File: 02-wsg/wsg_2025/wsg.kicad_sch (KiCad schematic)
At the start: 4 parts, among them J1 Conn_02x04_Counter_Clockwise, P1 USB_C_Plug_USB2.0, U5 ESP32-C6

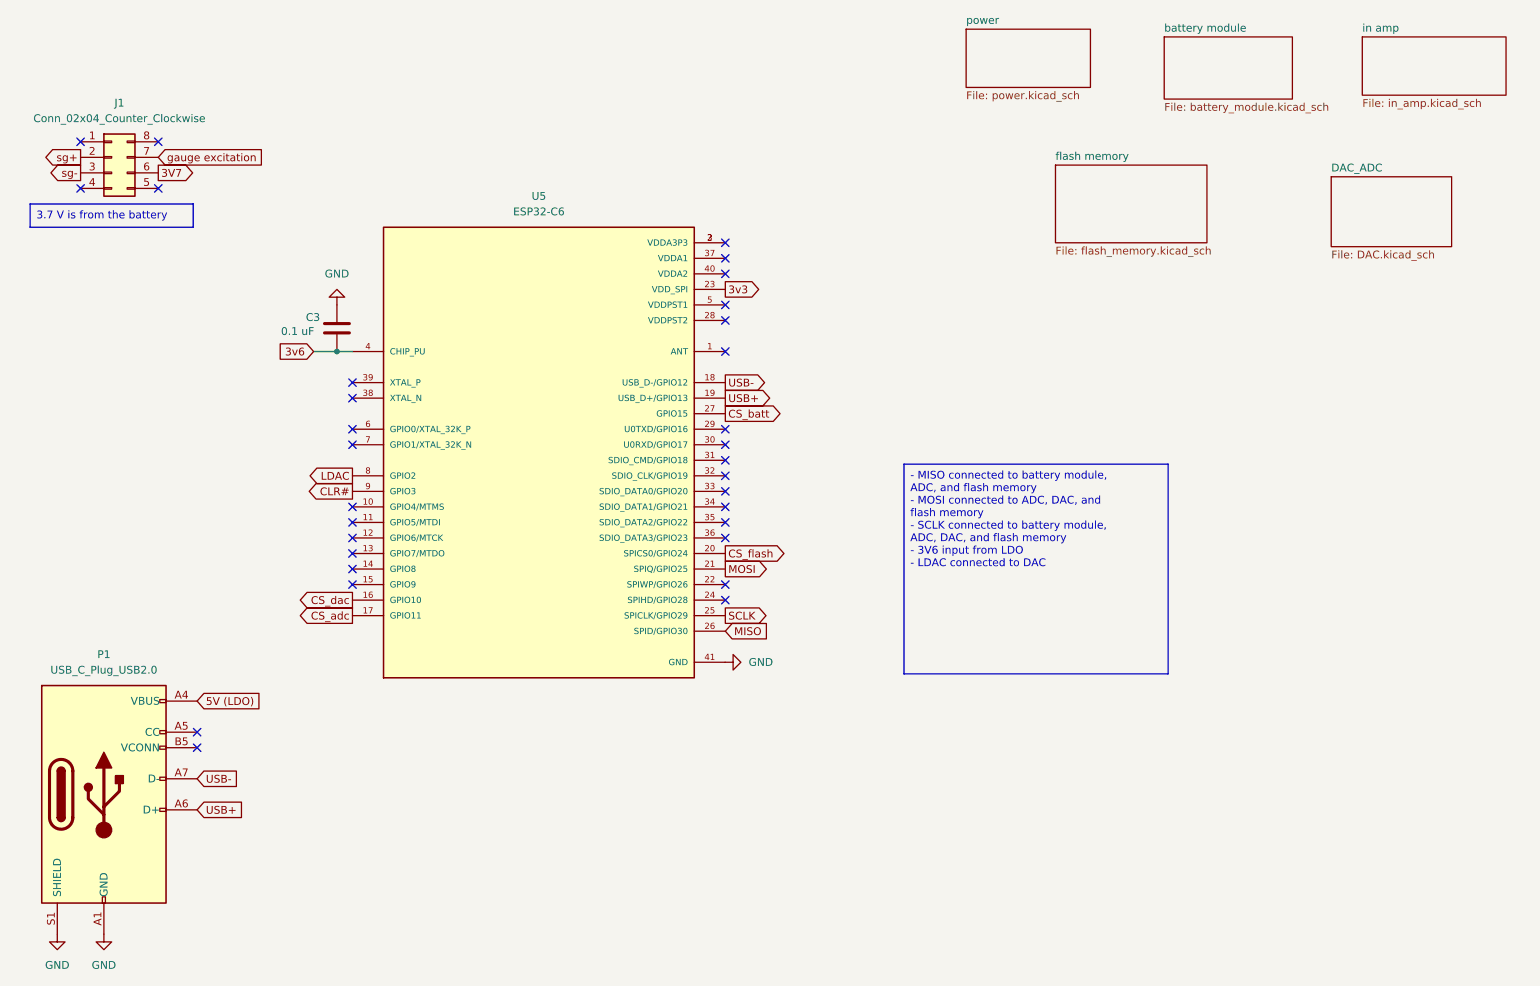
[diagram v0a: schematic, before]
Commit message: new wsg schem - not complete
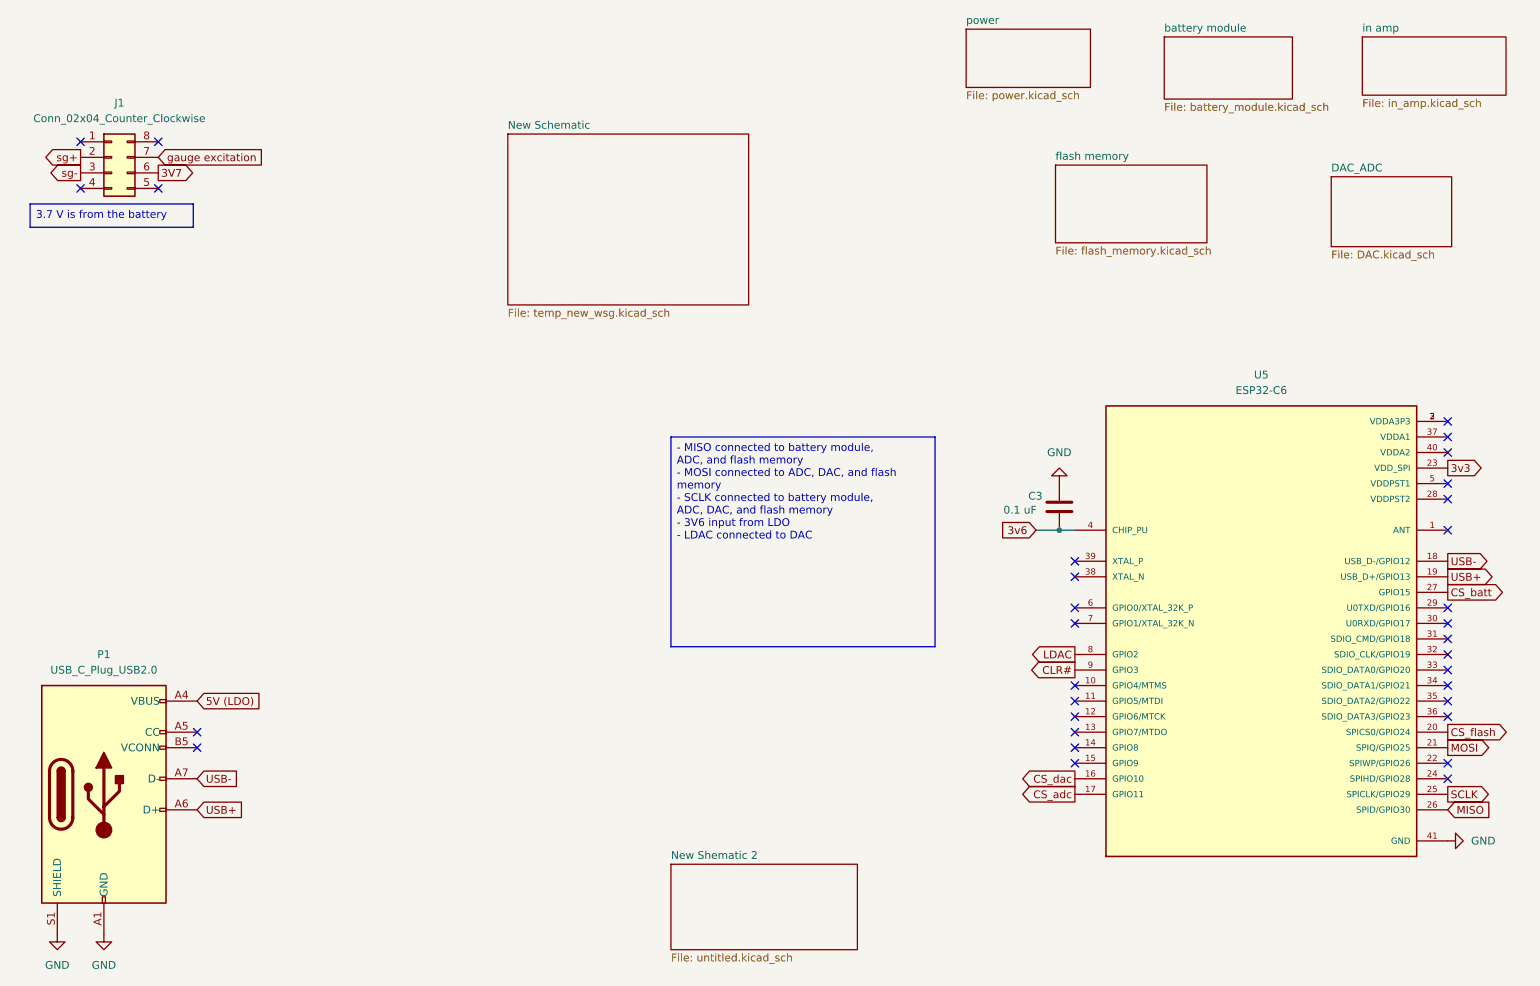
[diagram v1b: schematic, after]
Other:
- added sheet New Schematic (temp_new_wsg.kicad_sch)
- added sheet New Shematic 2 (untitled.kicad_sch)
- moved on the sheet: C3, U5
